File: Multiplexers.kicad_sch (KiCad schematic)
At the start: 7 parts

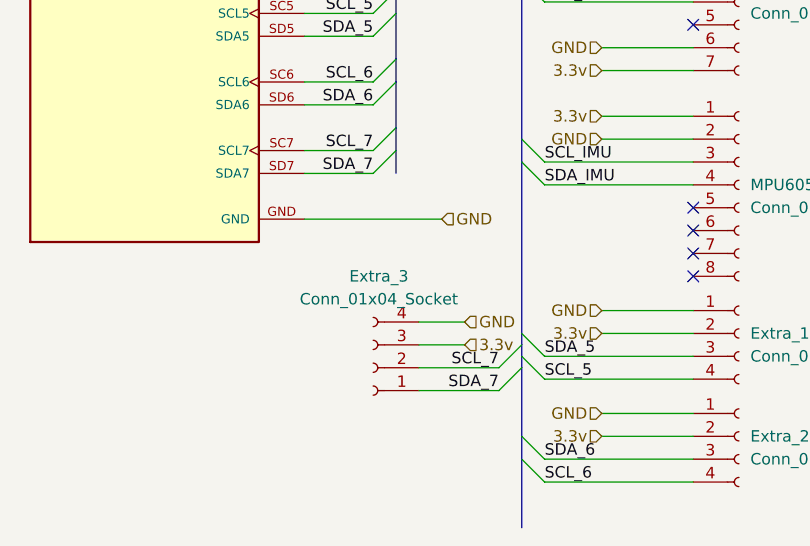
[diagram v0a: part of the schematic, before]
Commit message: erros ajustados e placa reformulada
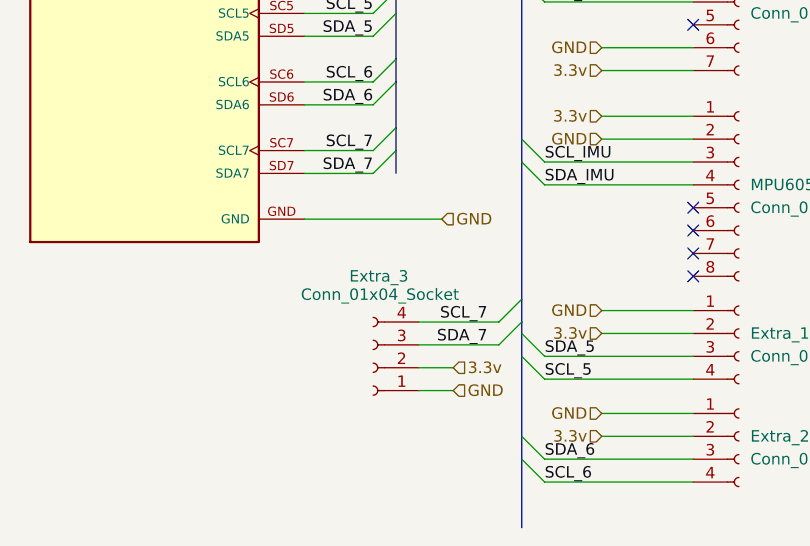
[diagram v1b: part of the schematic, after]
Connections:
- net 3.3v: now also Extra_3.2 (Pin_2); no longer Extra_3.3 (Pin_3)
- net GND: now also Extra_3.1 (Pin_1); no longer Extra_3.4 (Pin_4)
- net SCL_7: now also Extra_3.4 (Pin_4); no longer Extra_3.2 (Pin_2)
- net SDA_7: now also Extra_3.3 (Pin_3); no longer Extra_3.1 (Pin_1)
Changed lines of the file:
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@@
+	)
+	(bus_entry
+		(at 238.76 140.97)
+		(size -2.54 2.54)
+		(stroke
+			(width 0)
+			(type default)
+		)
 	)
 	(bus_entry
@@
 	)
 	(bus_entry
-		(at 238.76 146.05)
+		(at 238.76 138.43)
 		(size -2.54 2.54)
 		(stroke
@@
 	)
 	(bus_entry
-		(at 238.76 143.51)
-		(size -2.54 2.54)
-		(stroke
-			(width 0)
-			(type default)
-		)
-	)
-	(bus_entry
 		(at 238.76 81.28)
 		(size 2.54 2.54)
@@
 	(bus
 		(pts
-			(xy 238.76 123.19) (xy 238.76 142.24)
+			(xy 238.76 138.43) (xy 238.76 140.97)
+		)
+		(stroke
+			(width 0)
+			(type default)
+		)
+	)
+	(bus
+		(pts
+			(xy 238.76 123.19) (xy 238.76 138.43)
 		)
 		(stroke
@@
 	(wire
 		(pts
+			(xy 227.33 146.05) (xy 231.14 146.05)
+		)
+		(stroke
+			(width 0)
+			(type default)
+		)
+	)
+	(wire
+		(pts
 			(xy 241.3 147.32) (xy 257.81 147.32)
 		)
@@
 	(bus
 		(pts
-			(xy 238.76 143.51) (xy 238.76 144.78)
+			(xy 238.76 142.24) (xy 238.76 144.78)
 		)
 		(stroke
@@
 	(bus
 		(pts
-			(xy 238.76 144.78) (xy 238.76 146.05)
+			(xy 238.76 144.78) (xy 238.76 153.67)
 		)
 		(stroke
@@
 	(wire
 		(pts
-			(xy 227.33 140.97) (xy 232.41 140.97)
-		)
-		(stroke
-			(width 0)
-			(type default)
-		)
-	)
-	(wire
-		(pts
 			(xy 247.65 118.11) (xy 257.81 118.11)
 		)
@@
 	(bus
 		(pts
-			(xy 238.76 142.24) (xy 238.76 143.51)
-		)
-		(stroke
-			(width 0)
-			(type default)
-		)
-	)
-	(bus
-		(pts
 			(xy 238.76 156.21) (xy 238.76 163.83)
 		)
@@
 		)
 	)
+	(bus
+		(pts
+			(xy 238.76 140.97) (xy 238.76 142.24)
+		)
+		(stroke
+			(width 0)
+			(type default)
+		)
+	)
 	(wire
 		(pts
@@
 	(wire
 		(pts
-			(xy 227.33 146.05) (xy 236.22 146.05)
-		)
-		(stroke
-			(width 0)
-			(type default)
-		)
-	)
-	(wire
-		(pts
 			(xy 214.63 124.46) (xy 222.25 124.46)
 		)
@@
 	(wire
 		(pts
-			(xy 227.33 143.51) (xy 232.41 143.51)
-		)
-		(stroke
-			(width 0)
-			(type default)
-		)
-	)
-	(wire
-		(pts
 			(xy 175.26 73.66) (xy 175.26 76.2)
 		)
@@
 	(wire
 		(pts
+			(xy 227.33 143.51) (xy 236.22 143.51)
+		)
+		(stroke
+			(width 0)
+			(type default)
+		)
+	)
+	(wire
+		(pts
 			(xy 241.3 123.19) (xy 257.81 123.19)
 		)
@@
 		)
 	)
+	(wire
+		(pts
+			(xy 227.33 140.97) (xy 236.22 140.97)
+		)
+		(stroke
+			(width 0)
+			(type default)
+		)
+	)
 	(bus
 		(pts
@@
 		)
 	)
-	(bus
-		(pts
-			(xy 238.76 146.05) (xy 238.76 153.67)
+	(wire
+		(pts
+			(xy 227.33 148.59) (xy 231.14 148.59)
 		)
 		(stroke
@@
 		(pts
 			(xy 175.26 73.66) (xy 179.07 73.66)
-		)
-		(stroke
-			(width 0)
-			(type default)
-		)
-	)
-	(wire
-		(pts
-			(xy 227.33 148.59) (xy 236.22 148.59)
 		)
 		(stroke
@@
 	)
 	(label "SCL_7"
-		(at 236.22 146.05 180)
+		(at 234.95 140.97 180)
 		(effects
 			(font
@@
 	)
 	(label "SDA_7"
-		(at 236.22 148.59 180)
+		(at 234.95 143.51 180)
 		(effects
 			(font
@@
 	(hierarchical_label "3.3v"
 		(shape input)
-		(at 232.41 143.51 0)
+		(at 231.14 146.05 0)
 		(effects
 			(font
@@
 	(hierarchical_label "GND"
 		(shape input)
-		(at 232.41 140.97 0)
+		(at 231.14 148.59 0)
 		(effects
 			(font
@@
 		(on_board yes)
 		(dnp no)
-		(fields_autoplaced yes)
 		(property "Reference" "Extra_3"
 			(at 222.885 135.89 0)
@@
 		)
 		(property "Value" "Conn_01x04_Socket"
-			(at 222.885 138.43 0)
+			(at 223.012 137.922 0)
 			(effects
 				(font
